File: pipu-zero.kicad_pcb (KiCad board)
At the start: 4 copper layers, 80 x 50.5 mm, 80 parts, among them IC1 BQ25176JDSGR, J1 USB_C_Receptacle_USB2.0_14P, J2 Conn_01x08, J3 Micro_SD_Card_Det1, Q1 NMOS, Q2 NMOS, Q3 NMOS, Q4 NMOS, SW1 SW_Push, SW2 SW_Push, U1 BQ297xy, U2 MCP1640Bx-xCHY, U3 MCP1727-0802xSN, U4 ESP32-S3-WROOM-1, U5 CC1101, U6 DM-OLED096-636, U7 TSOP348xx, Y2 Crystal_GND23

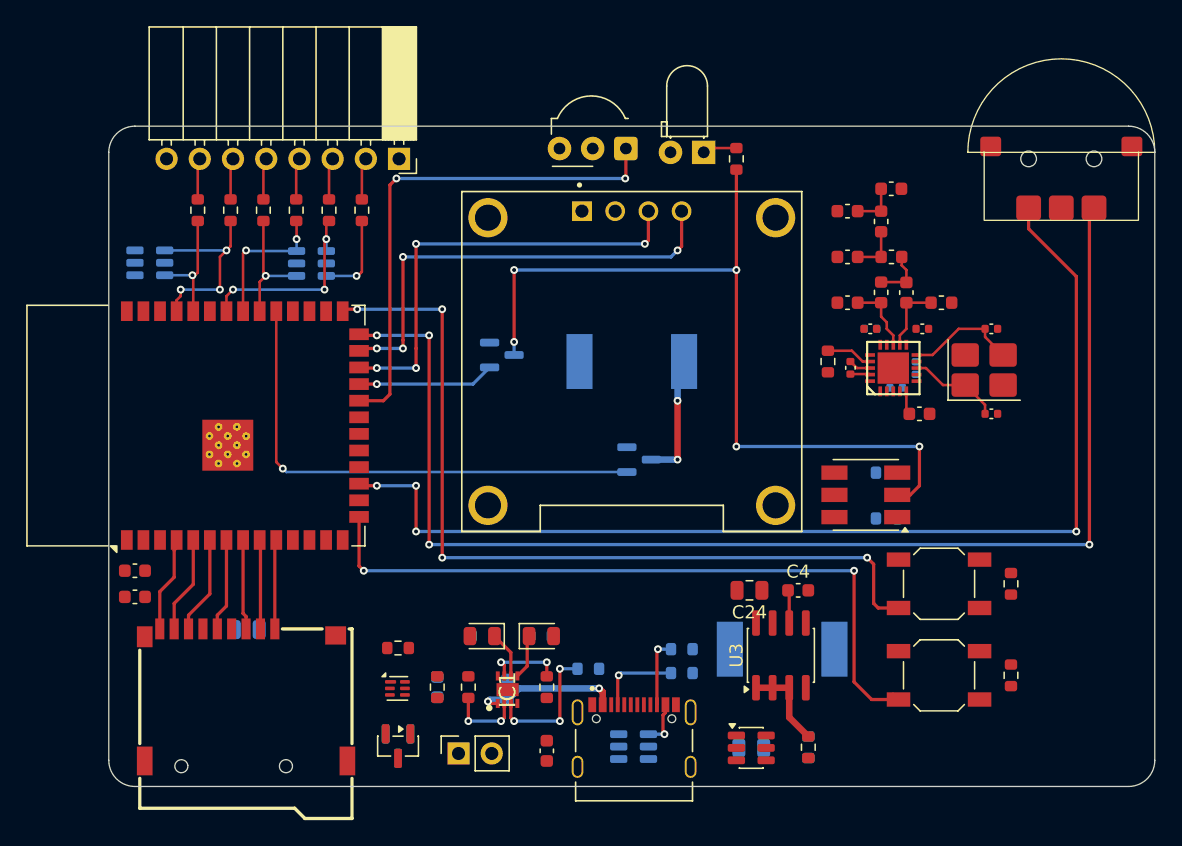
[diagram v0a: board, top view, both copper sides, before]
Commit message: routing
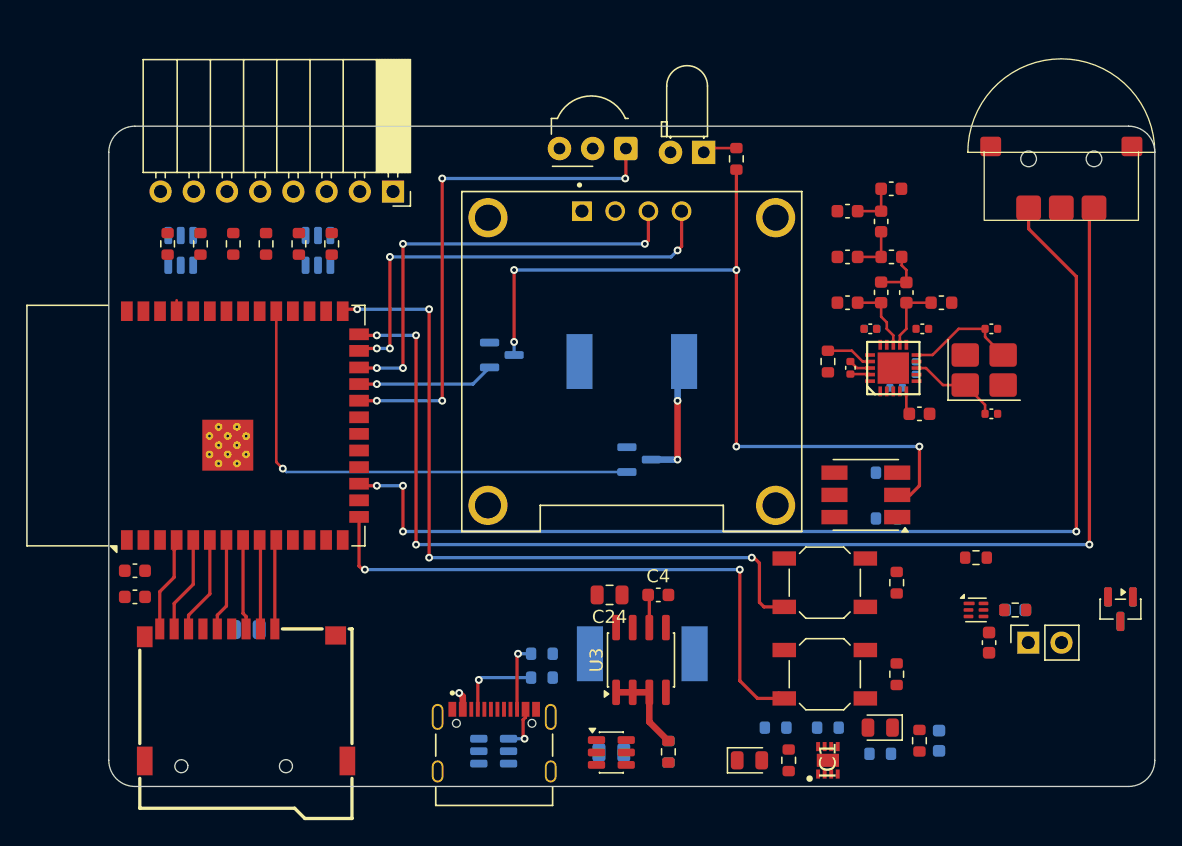
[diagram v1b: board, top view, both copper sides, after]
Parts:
- moved Q1 56.2 mm to (190.9, 99.4)
- moved Q2 56.2 mm to (190.9, 99.4)
- moved R7 44.7 mm to (179.8, 95.5)
- moved U1 44.7 mm to (179.8, 99.5)
- moved C2 44.6 mm to (182.8, 99.5), turned to 0 degrees
- moved R3 44.6 mm to (182.8, 99.5), turned to 180 degrees
- moved BT1 44.4 mm to (183.8, 102.0)
- moved C3 34.8 mm to (180.8, 102.0), turned to -90 degrees
- moved C1 33.2 mm to (177.0, 109.5)
- moved D3 31.2 mm to (172.5, 108.5)
- moved R8 28.8 mm to (175.5, 109.5)
- moved R4 25.1 mm to (165.5, 111.0)
- moved IC1 25.1 mm to (168.5, 111.0)
- moved R6 23.5 mm to (164.5, 108.5)
- moved R19 23.3 mm to (172.5, 110.5)
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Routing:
- net /I-O/IO41: track 15.2 -> 0.00 mm, vias 3 -> 0
- net /I-O/TXD0: track 15.1 -> 0.84 mm, vias 3 -> 0
- net /I-O/IO40: track 10.9 -> 0.00 mm, vias 2 -> 0
- net /Power Manager/BAT_NTC: track 10.3 -> 0.00 mm, vias 3 -> 0
- net /USB_VBUS: track 14.9 -> 4.96 mm, vias 3 -> 2
- net /I-O/IO39: track 9.53 -> 0.00 mm, vias 1 -> 0
- net /I-O/RXD0: track 9.33 -> 0.00 mm, vias 1 -> 0
- net /I-O/BTN2: track 54.8 -> 46.0 mm
- net /I-O/BTN1: track 64.9 -> 56.2 mm
- net /I-O/IO42: track 6.74 -> 0.00 mm, vias 1 -> 0
- net Net-(IC1-VSET): track 5.73 -> 0.00 mm, vias 2 -> 0
- net Net-(IC1-ISET): track 5.73 -> 0.00 mm, vias 2 -> 0
- net Net-(D3-K): track 3.57 -> 0.00 mm
- net Net-(D2-K): track 3.42 -> 0.00 mm
- net /I-O/IO42_EXT: track 3.23 -> 0.00 mm
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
